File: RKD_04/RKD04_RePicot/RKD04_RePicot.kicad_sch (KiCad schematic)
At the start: 6 parts, among them J1 TRRS, J2 Conn_01x24, J3 Qwiic_RA, J4 Conn_01x06, U1 Pico

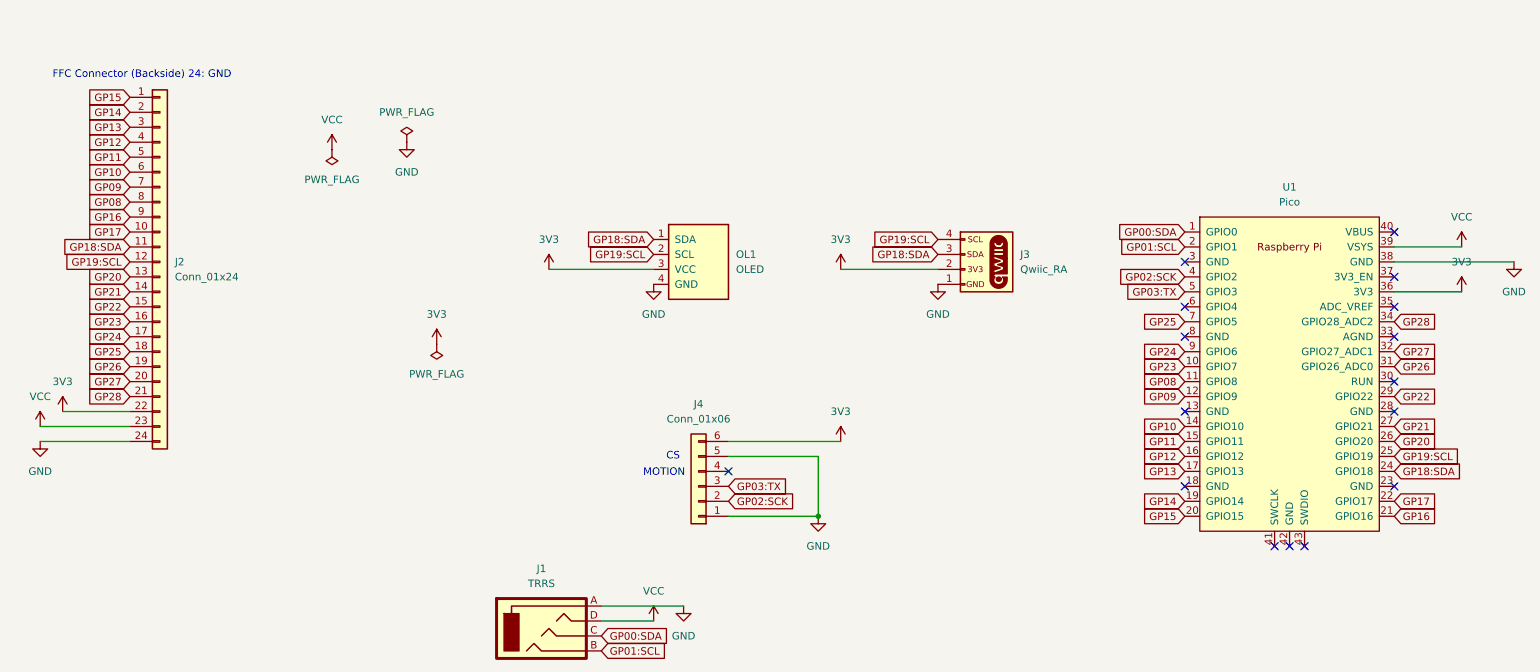
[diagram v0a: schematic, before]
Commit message: Modify for SekiBall
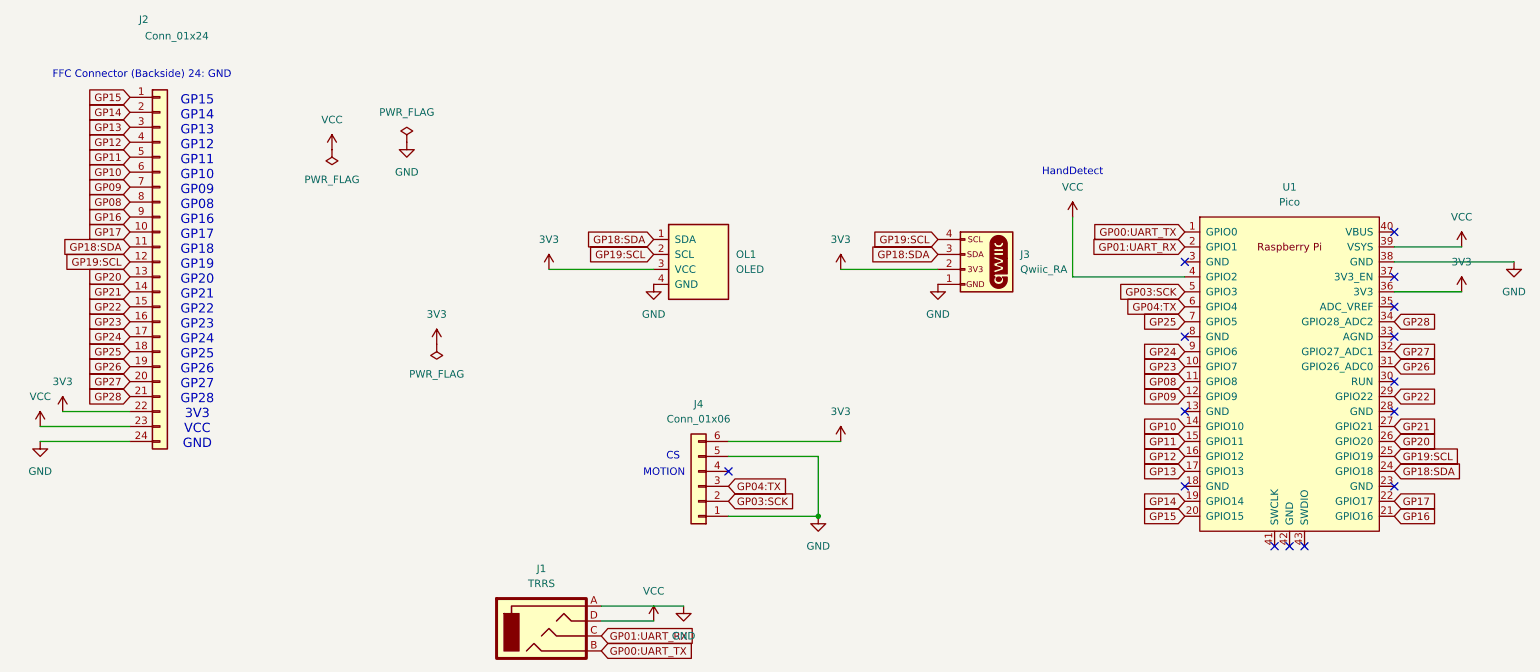
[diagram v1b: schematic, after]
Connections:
- net VCC: now also U1.4 (GPIO2)
- net GP04:TX: now reaches U1.6 (GPIO4)
- net GP04:TX: now also J4.3 (Pin_3)
- net GP00:SDA renamed GP00:UART_TX
- net GP00:UART_TX: now also J1.B; no longer J1.C
- net GP01:SCL renamed GP01:UART_RX
- net GP01:UART_RX: now also J1.C; no longer J1.B
- net GP02:SCK renamed GP03:SCK
- net GP03:SCK: now also U1.5 (GPIO3); no longer U1.4 (GPIO2)
- removed net GP03:TX: J4.3 (Pin_3), U1.5 (GPIO3)
- no-connect marks 16 -> 15
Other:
- note added: "GP15 GP14 GP13 GP12 GP11 GP10 GP09 GP08 GP16 GP17 GP18 GP19 GP20 GP21 GP22 GP23 GP24 GP25 GP26 GP27 GP28 3V3 VCC GND"
- note added: "HandDetect"

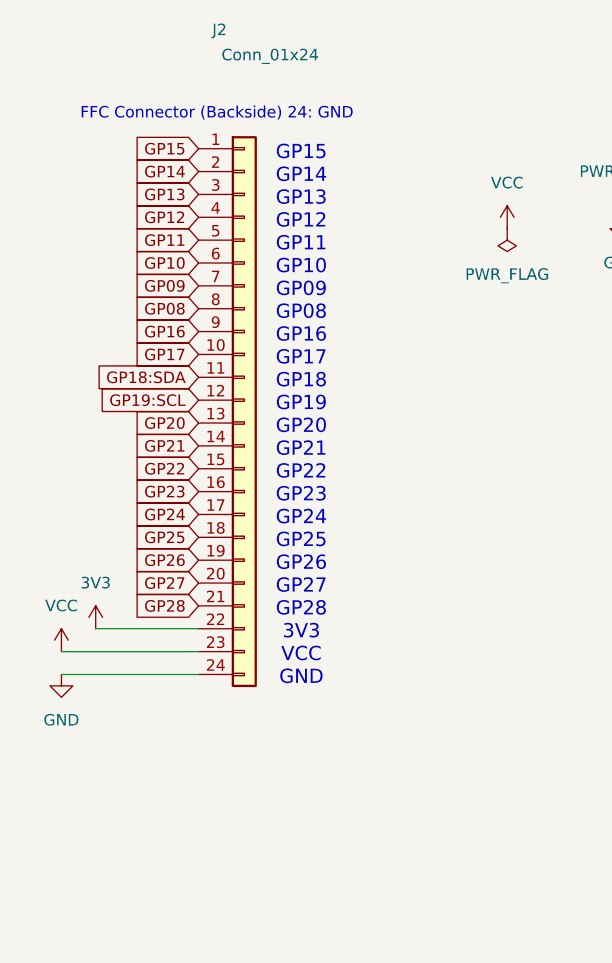
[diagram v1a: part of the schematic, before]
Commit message: RePicotの修正
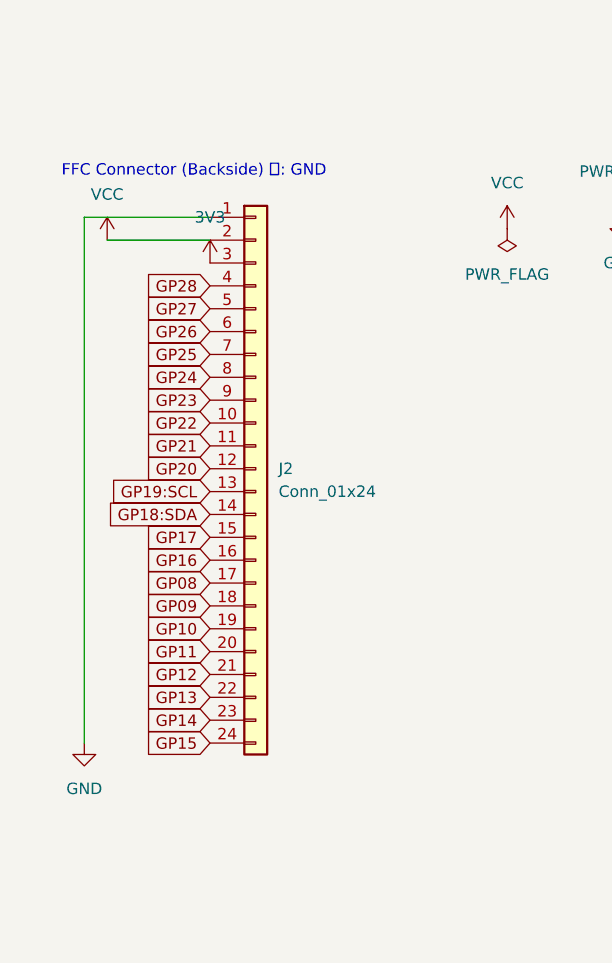
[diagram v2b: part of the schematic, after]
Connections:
- net 3V3: now also J2.3 (Pin_3); no longer J2.22 (Pin_22)
- net GND: now also J2.1 (Pin_1); no longer J2.24 (Pin_24)
- net GP08: now also J2.17 (Pin_17); no longer J2.8 (Pin_8)
- net GP09: now also J2.18 (Pin_18); no longer J2.7 (Pin_7)
- net GP10: now also J2.19 (Pin_19); no longer J2.6 (Pin_6)
- net GP11: now also J2.20 (Pin_20); no longer J2.5 (Pin_5)
- net GP12: now also J2.21 (Pin_21); no longer J2.4 (Pin_4)
- net GP13: now also J2.22 (Pin_22); no longer J2.3 (Pin_3)
- net GP14: now also J2.23 (Pin_23); no longer J2.2 (Pin_2)
- net GP15: now also J2.24 (Pin_24); no longer J2.1 (Pin_1)
- net GP16: now also J2.16 (Pin_16); no longer J2.9 (Pin_9)
- net GP17: now also J2.15 (Pin_15); no longer J2.10 (Pin_10)
- net GP18:SDA: now also J2.14 (Pin_14); no longer J2.11 (Pin_11)
- net GP19:SCL: now also J2.13 (Pin_13); no longer J2.12 (Pin_12)
- net GP20: now also J2.12 (Pin_12); no longer J2.13 (Pin_13)
- net GP21: now also J2.11 (Pin_11); no longer J2.14 (Pin_14)
- net GP22: now also J2.10 (Pin_10); no longer J2.15 (Pin_15)
- net GP23: now also J2.9 (Pin_9); no longer J2.16 (Pin_16)
- net GP24: now also J2.8 (Pin_8); no longer J2.17 (Pin_17)
- net GP25: now also J2.7 (Pin_7); no longer J2.18 (Pin_18)
- net GP26: now also J2.6 (Pin_6); no longer J2.19 (Pin_19)
- net GP27: now also J2.5 (Pin_5); no longer J2.20 (Pin_20)
- net GP28: now also J2.4 (Pin_4); no longer J2.21 (Pin_21)
- net VCC: now also J2.2 (Pin_2); no longer J2.23 (Pin_23)
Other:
- note added: "FFC Connector (Backside) １: GND"
- note removed: "FFC Connector (Backside) 24: GND"
- note removed: "GP15 GP14 GP13 GP12 GP11 GP10 GP09 GP08 GP16 GP17 GP18 GP19 GP20 GP21 GP22 GP23 GP24 GP25 GP26 GP27 GP28 3V3 VCC GND"
